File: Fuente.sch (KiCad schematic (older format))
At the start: 22 parts, among them U201 XL4005E1, U202 XL4005E1

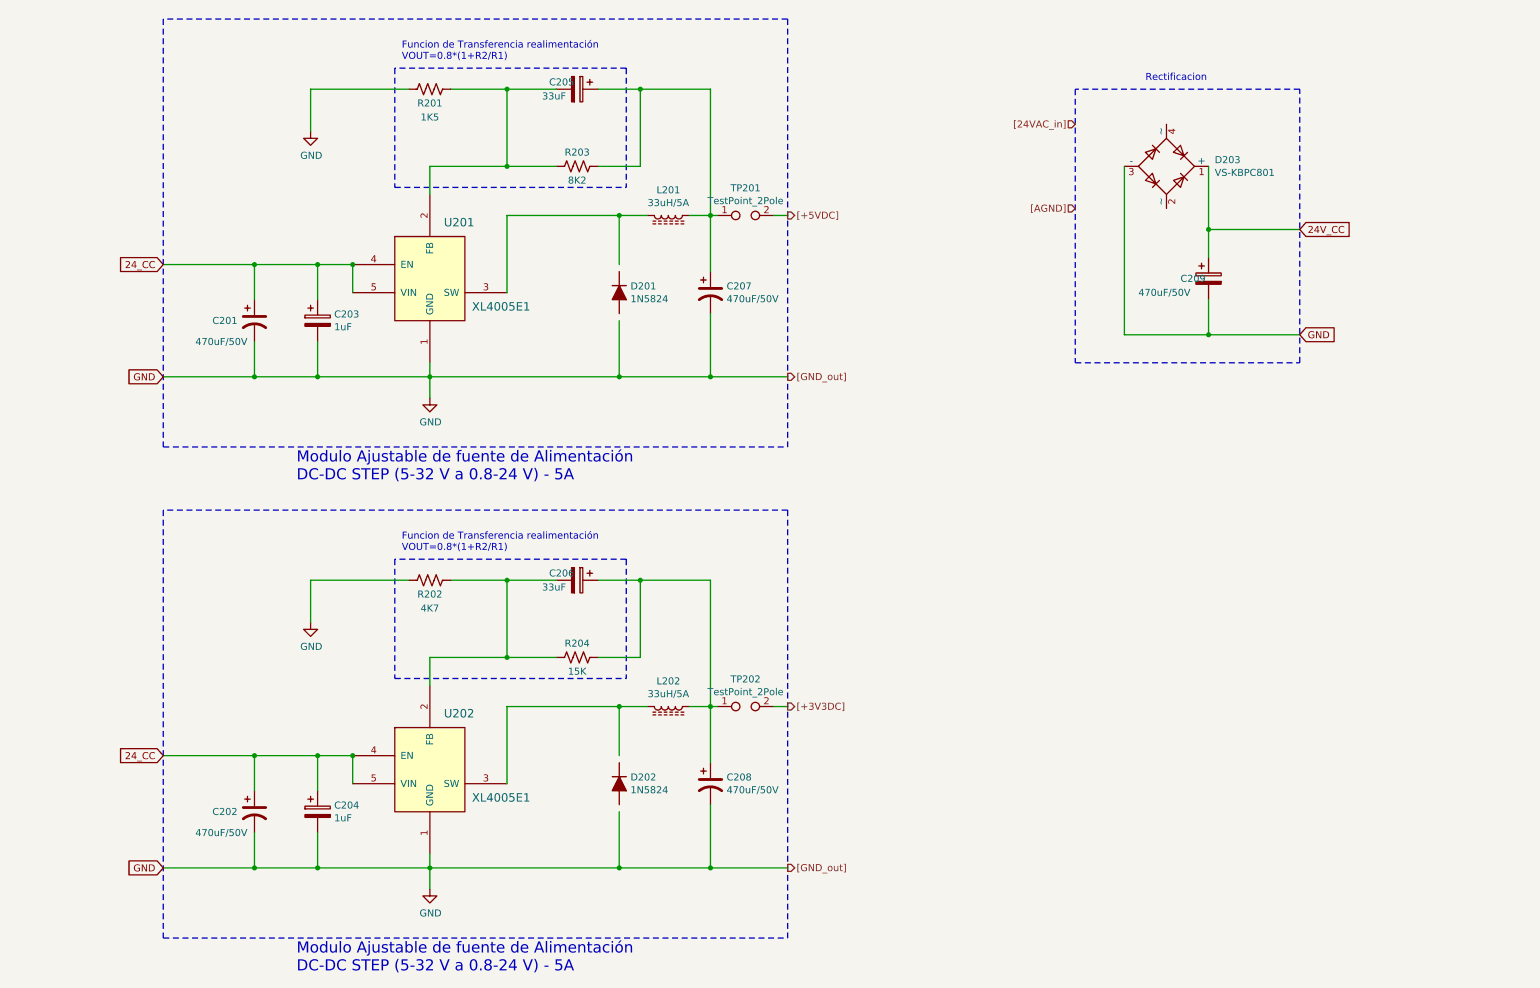
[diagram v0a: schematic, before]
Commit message: Agrego v1.0 de SmartSaffron
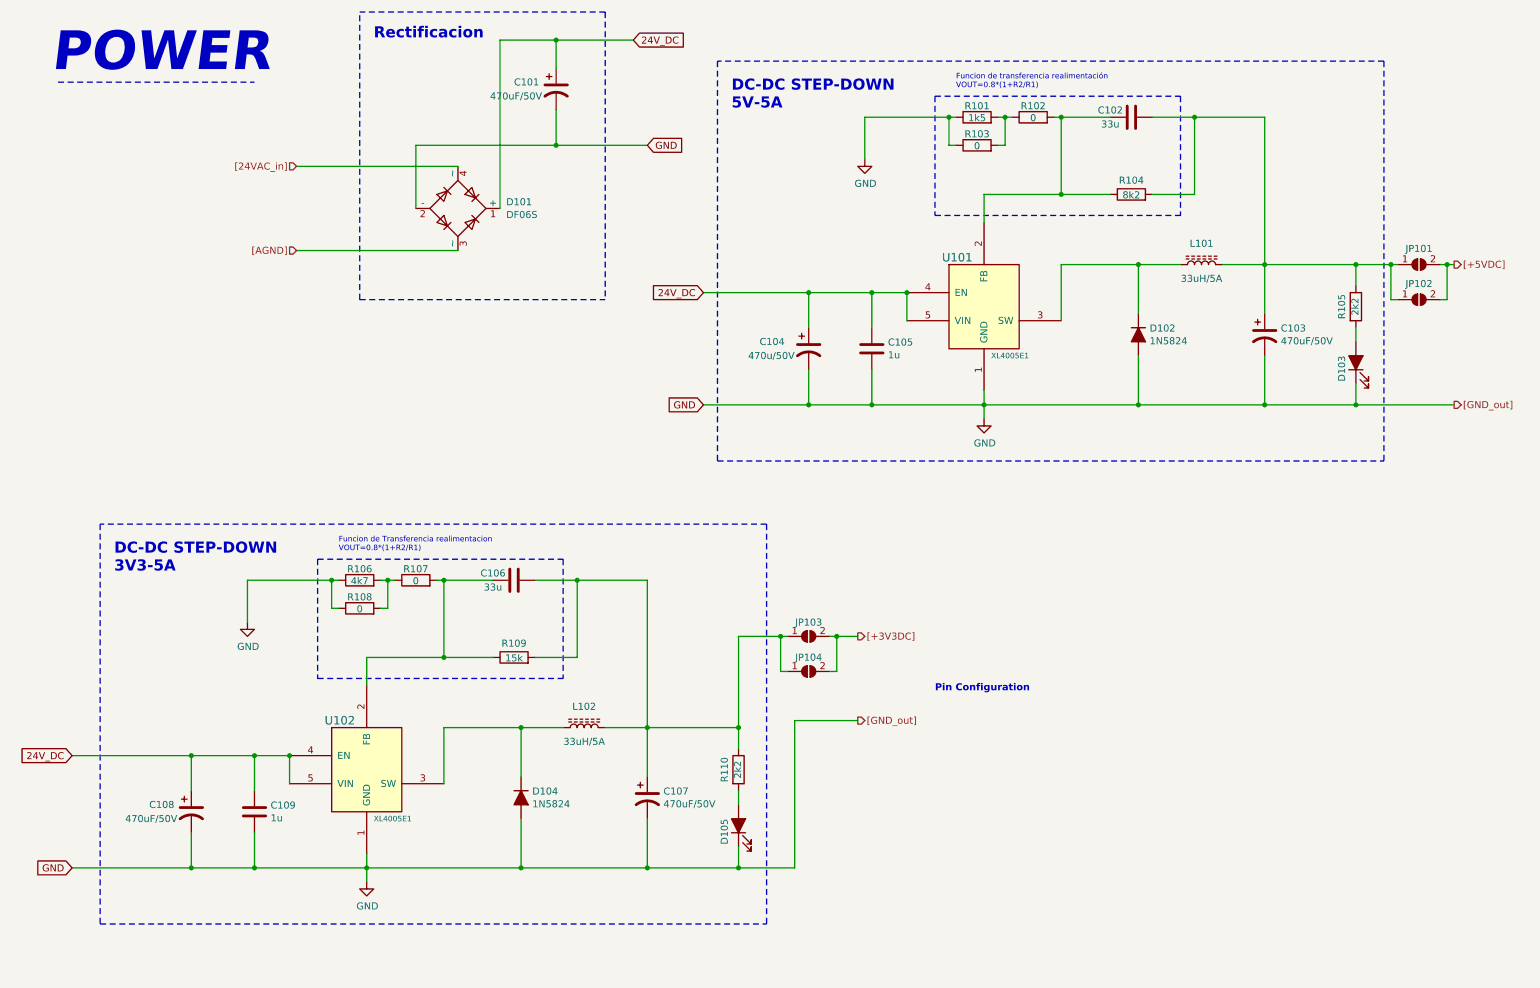
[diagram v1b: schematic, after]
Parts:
- removed C203, C204: 1uF, symbol Device:CP
- removed C205, C206: 33uF, symbol Device:CP
- removed C209: 470uF/50V, symbol Device:CP
- removed D203: VS-KBPC801, Diode_THT:Diode_Bridge_Vishay_KBPC6, symbol Diode_Bridge:VS-KBPC801
- removed R201: 1K5, symbol Device:R_US
- removed R202: 4K7, symbol Device:R_US
- removed R203: 8K2, symbol Device:R_US
- removed R204: 15K, symbol Device:R_US
- removed TP201, TP202: TestPoint_2Pole, symbol Connector:TestPoint_2Pole
- added C101: 470uF/50V, 00_lib_fp:CP_Elec_10x10, symbol Device:CP1
- added C102, C106: 33u, 00_lib_fp:C_0805_2012Metric_Pad1.18x1.45mm_HandSolder, symbol 00_lib_sch:C
- added C105, C109: 1u, 00_lib_fp:C_0805_2012Metric_Pad1.18x1.45mm_HandSolder, symbol 00_lib_sch:C
- added D101: DF06S, 00_lib_fp:Diode_Bridge_Vishay_DFSFlat, symbol 00_lib_sch:DF06S
- added D103, D105: green, 00_lib_fp:LED_0805_2012Metric_Castellated, symbol 00_lib_sch:LED_ALT
- added JP101, JP102, JP103, JP104: jumper, 00_lib_fp:SolderJumper-2_P1.3mm_Open_RoundedPad1.0x1.5mm, symbol 00_lib_sch:jumper
- added R101: 1k5, 00_lib_fp:R_0805_2012Metric_Pad1.20x1.40mm_HandSolder, symbol 00_lib_sch:R
- added R102, R103, R107, R108: 0, 00_lib_fp:R_0805_2012Metric_Pad1.20x1.40mm_HandSolder, symbol 00_lib_sch:R
- added R104: 8k2, 00_lib_fp:R_0805_2012Metric_Pad1.20x1.40mm_HandSolder, symbol 00_lib_sch:R
- added R105, R110: 2k2, 00_lib_fp:R_0805_2012Metric_Pad1.20x1.40mm_HandSolder, symbol 00_lib_sch:R
- added R106: 4k7, 00_lib_fp:R_0805_2012Metric_Pad1.20x1.40mm_HandSolder, symbol 00_lib_sch:R
- added R109: 15k, 00_lib_fp:R_0805_2012Metric_Pad1.20x1.40mm_HandSolder, symbol 00_lib_sch:R
- C103: renamed from C207; footprint (none) -> 00_lib_fp:CP_Elec_8x10.5
- C104: renamed from C201; value 470uF/50V -> 470u/50V; footprint (none) -> 00_lib_fp:CP_Elec_8x10.5
- C107: renamed from C208; footprint (none) -> 00_lib_fp:CP_Elec_8x10.5
- C108: renamed from C202; footprint (none) -> 00_lib_fp:CP_Elec_8x10.5
- D102: renamed from D201; footprint DIOAD1898W129L762D1143 -> 00_lib_fp:D_SMB_Handsoldering
- D104: renamed from D202; footprint DIOAD1898W129L762D1143 -> 00_lib_fp:D_SMB_Handsoldering
- L101: renamed from L201; footprint (none) -> 00_lib_fp:Coil_ferrite
- L102: renamed from L202; footprint (none) -> 00_lib_fp:Coil_ferrite
- U101: renamed from U201; footprint (none) -> 00_lib_fp:TO-263-5_TabPin3
- U102: renamed from U202; footprint (none) -> 00_lib_fp:TO-263-5_TabPin3
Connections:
- net labels added: 24V_DC
- net labels removed: 24V_CC, 24_CC
- wire segments 85 -> 127
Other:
- note added: "DC-DC STEP-DOWN \n3V3-5A"
- note added: "DC-DC STEP-DOWN \n5V-5A"
- note added: "Funcion de Transferencia realimentacion\nVOUT=0.8*(1+R2/R1)"
- note added: "Funcion de transferencia realimentación\nVOUT=0.8*(1+R2/R1)"
- note added: "POWER"
- note added: "Pin Configuration"
- note removed: "Funcion de Transferencia realimentación\nVOUT=0.8*(1+R2/R1)"
- note removed: "Modulo Ajustable de fuente de Alimentación\nDC-DC STEP (5-32 V a 0.8-24 V) - 5A"
- moved on the sheet: C103, C104, C107, C108, D102, D104, L101, L102, U101, U102

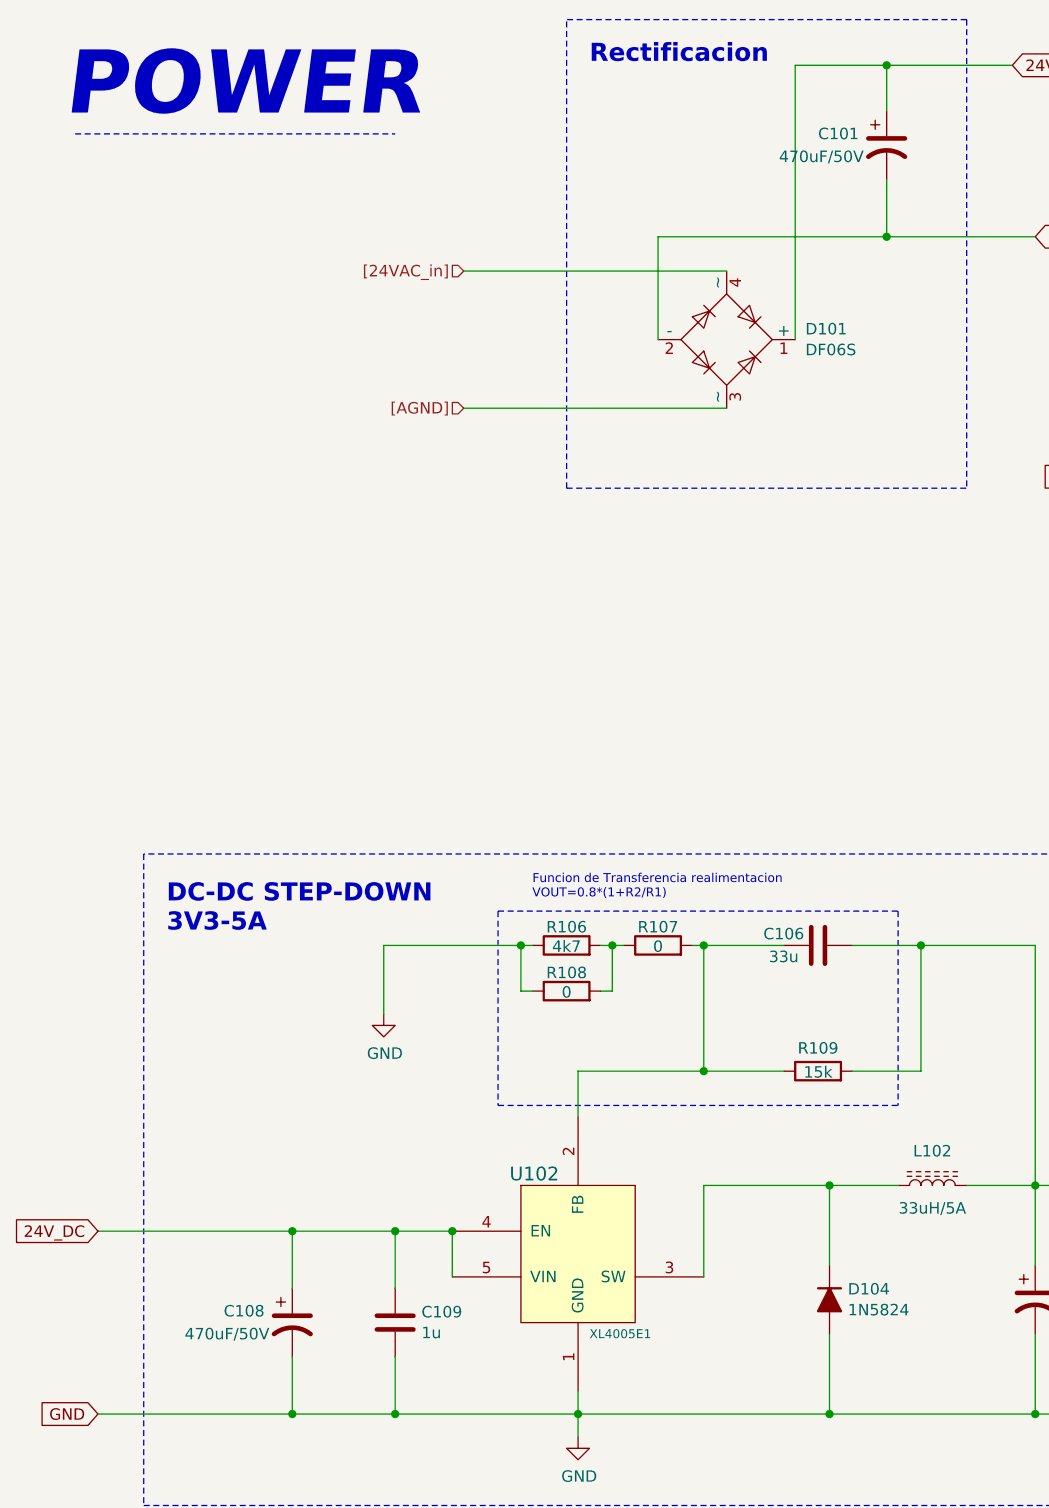
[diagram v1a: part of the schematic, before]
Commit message: Revision
    * Acomodo los datos de F.Fab y B.Fab
    * Genero ibom
    * Exporto PDF e imagenes
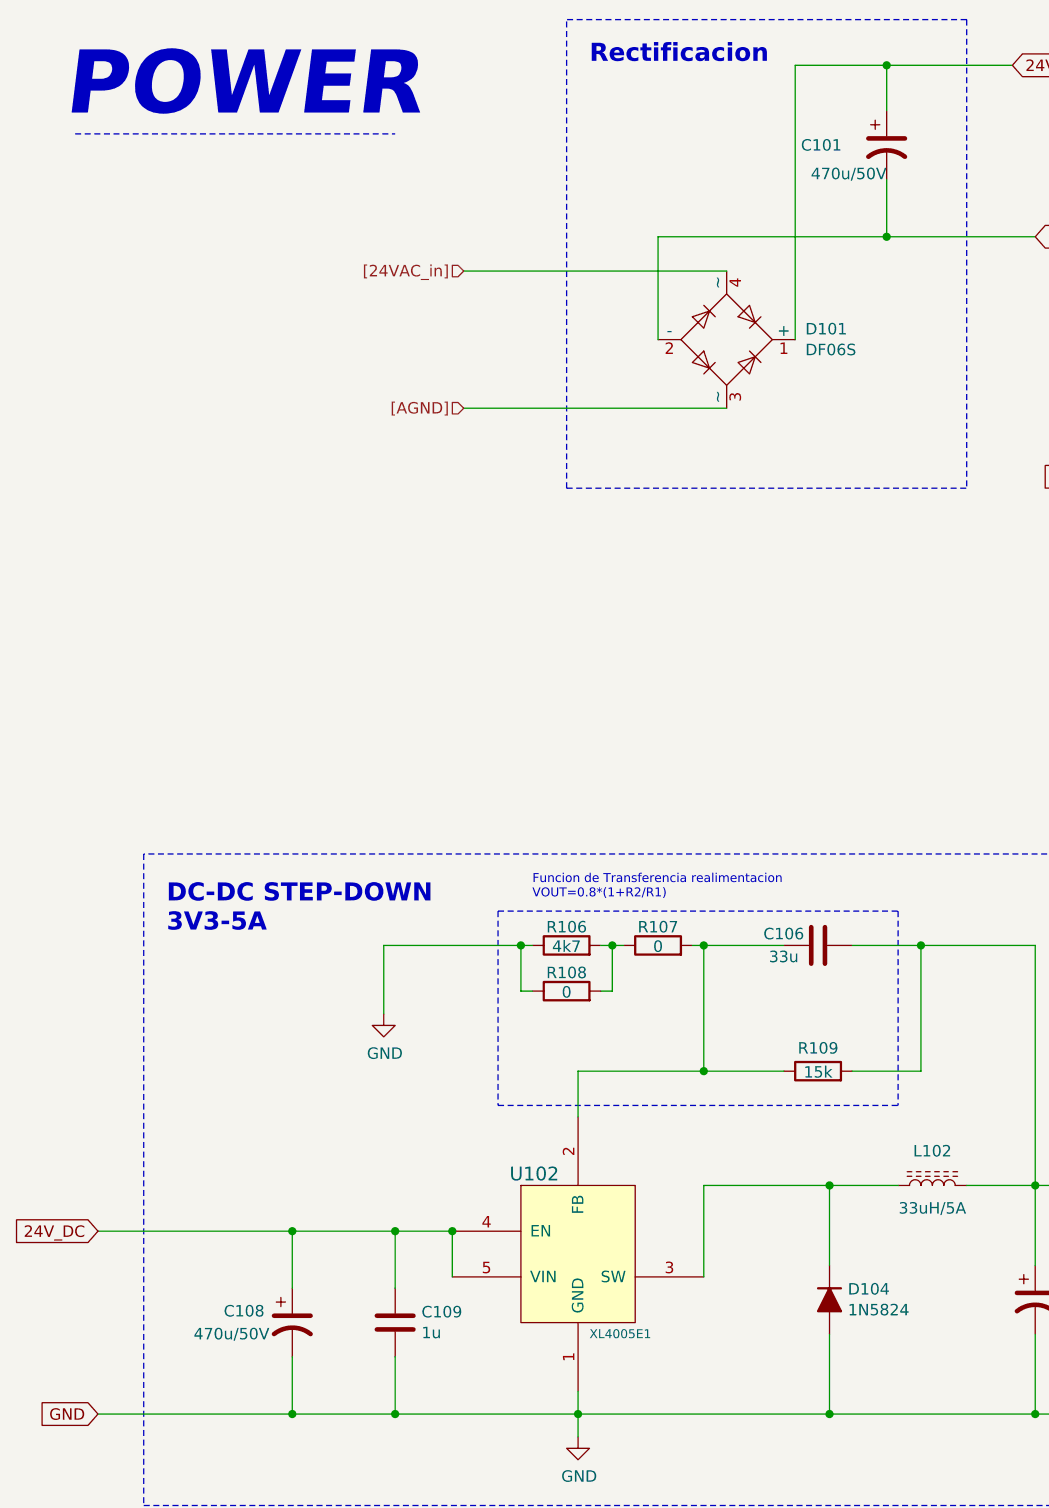
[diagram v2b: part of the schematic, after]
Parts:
- C101, C108: value 470uF/50V -> 470u/50V
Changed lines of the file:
@@
 P 1700 6400
 F 0 "C108" H 1400 6450 50  0000 L CNN
-F 1 "470uF/50V" H 1600 6350 50  0000 R CNN
+F 1 "470u/50V" H 1600 6350 50  0000 R CNN
 F 2 "00_lib_fp:CP_Elec_8x10.5" H 1700 6400 50  0001 C CNN
 F 3 "~" H 1700 6400 50  0001 C CNN
@@
 U 1 1 61A488D3
 P 4300 1250
-F 0 "C101" H 4000 1300 50  0000 L CNN
-F 1 "470uF/50V" H 4200 1200 50  0000 R CNN
+F 0 "C101" H 3925 1250 50  0000 L CNN
+F 1 "470u/50V" H 4300 1125 50  0000 R CNN
 F 2 "00_lib_fp:CP_Elec_10x10" H 4300 1250 50  0001 C CNN
 F 3 "~" H 4300 1250 50  0001 C CNN
